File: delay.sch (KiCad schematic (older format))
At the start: 19 parts, among them U201 PT2399

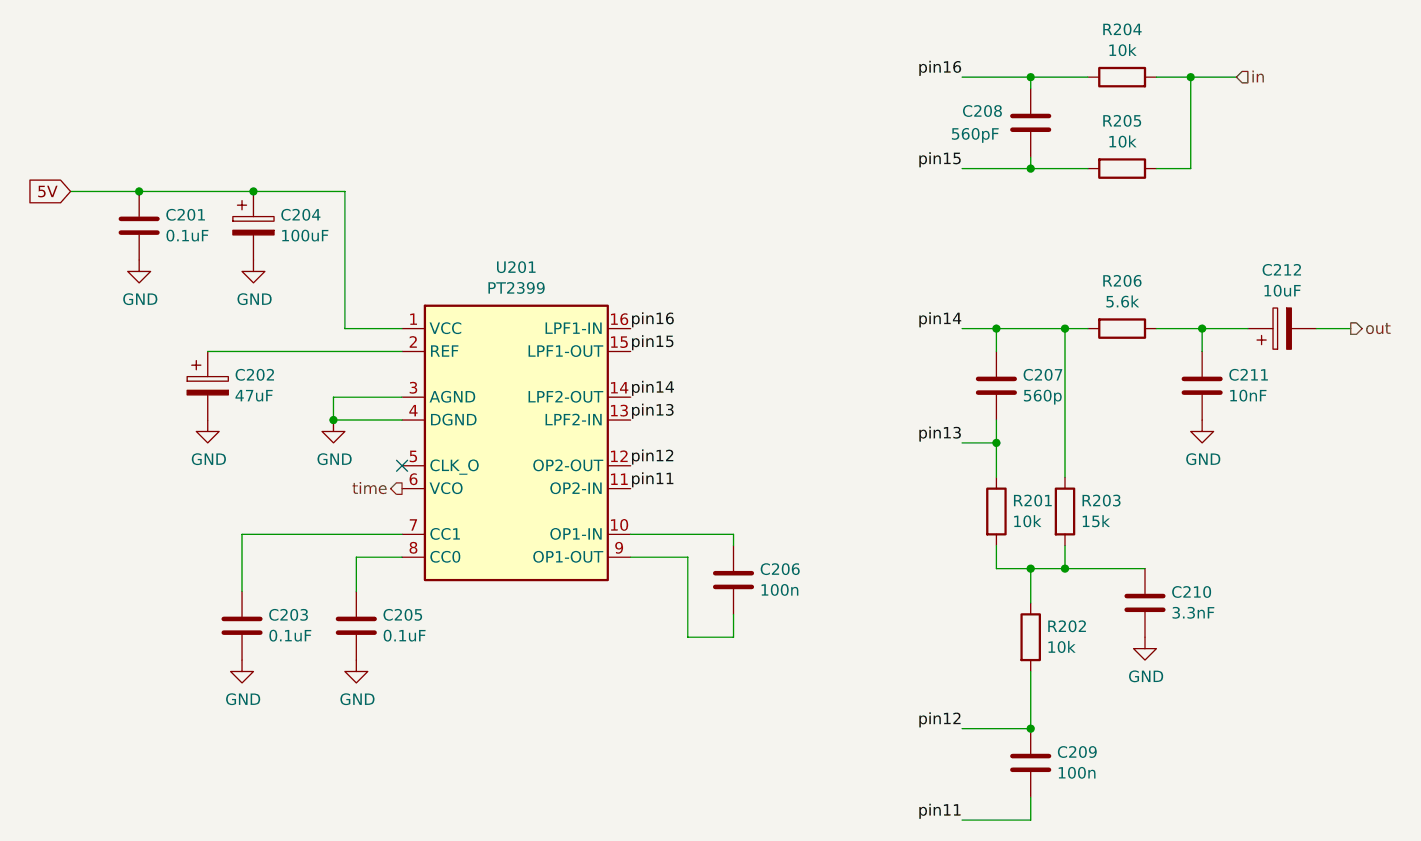
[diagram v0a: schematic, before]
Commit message: Clipping diodes work
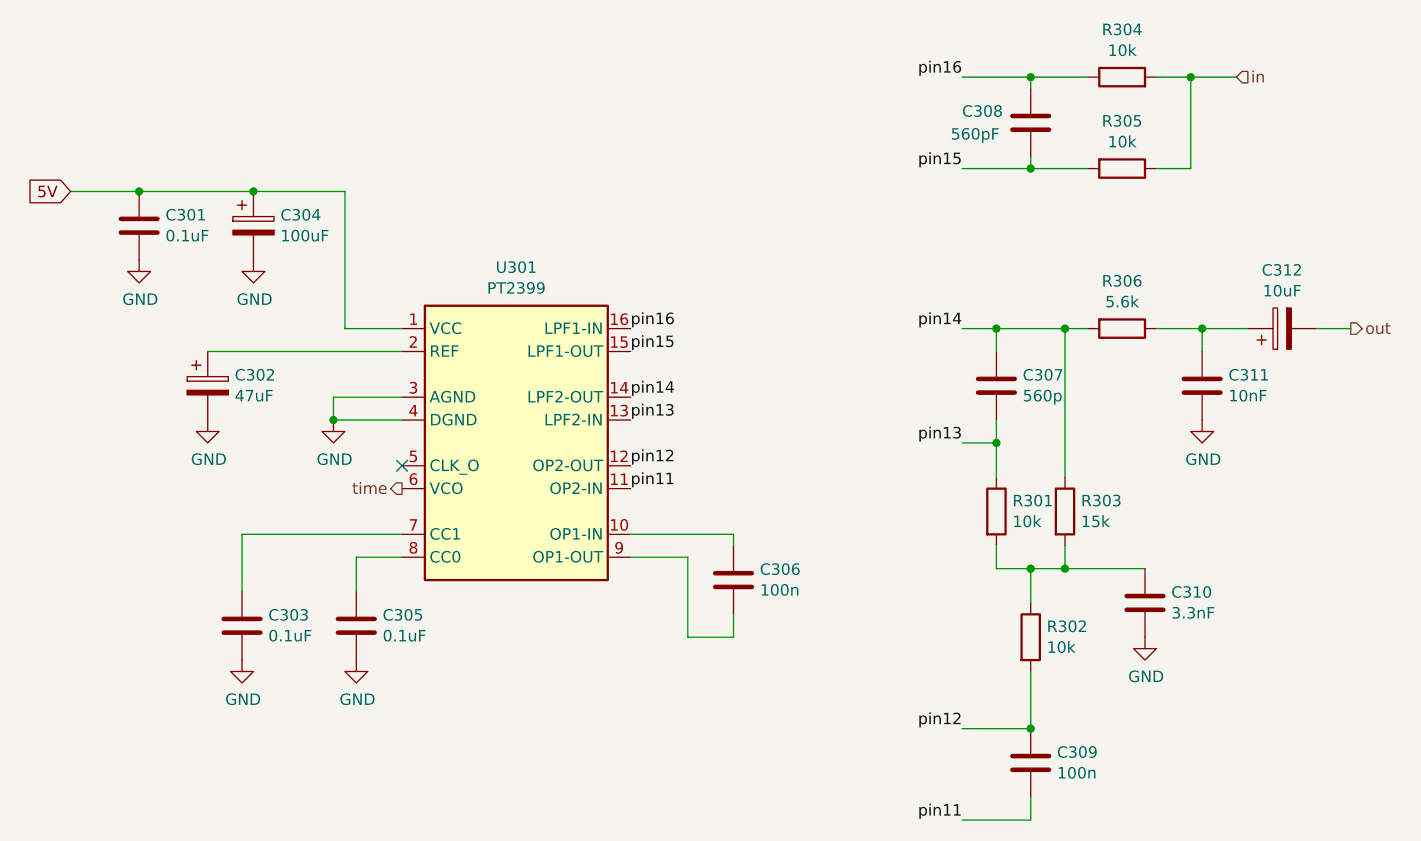
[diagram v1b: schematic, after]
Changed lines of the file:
@@
 AR Path="/5F90D1E6/5F9242A3" Ref="U201"  Part="1"
 AR Path="/5F9672E5/5F9242A3" Ref="U301"  Part="1"
-F 0 "U201" H 3700 4267 50  0000 C CNN
+F 0 "U301" H 3700 4267 50  0000 C CNN
 F 1 "PT2399" H 3700 4176 50  0000 C CNN
 F 2 "" H 3700 3100 50  0001 C CNN
@@
 AR Path="/5F90D1E6/5F9242A9" Ref="C203"  Part="1"
 AR Path="/5F9672E5/5F9242A9" Ref="C303"  Part="1"
-F 0 "C203" H 2615 4346 50  0000 L CNN
+F 0 "C303" H 2615 4346 50  0000 L CNN
 F 1 "0.1uF" H 2615 4255 50  0000 L CNN
 F 2 "" H 2538 4150 50  0001 C CNN
@@
 AR Path="/5F90D1E6/5F9242AF" Ref="C205"  Part="1"
 AR Path="/5F9672E5/5F9242AF" Ref="C305"  Part="1"
-F 0 "C205" H 3115 4346 50  0000 L CNN
+F 0 "C305" H 3115 4346 50  0000 L CNN
 F 1 "0.1uF" H 3115 4255 50  0000 L CNN
 F 2 "" H 3038 4150 50  0001 C CNN
@@
 AR Path="/5F90D1E6/5F9242B9" Ref="#PWR0204"  Part="1"
 AR Path="/5F9672E5/5F9242B9" Ref="#PWR0304"  Part="1"
-F 0 "#PWR0204" H 2500 4200 50  0001 C CNN
+F 0 "#PWR0304" H 2500 4200 50  0001 C CNN
 F 1 "GND" H 2505 4277 50  0000 C CNN
 F 2 "" H 2500 4450 50  0001 C CNN
@@
 AR Path="/5F90D1E6/5F9242BF" Ref="#PWR0207"  Part="1"
 AR Path="/5F9672E5/5F9242BF" Ref="#PWR0307"  Part="1"
-F 0 "#PWR0207" H 3000 4200 50  0001 C CNN
+F 0 "#PWR0307" H 3000 4200 50  0001 C CNN
 F 1 "GND" H 3005 4277 50  0000 C CNN
 F 2 "" H 3000 4450 50  0001 C CNN
@@
 AR Path="/5F90D1E6/5F9242C5" Ref="C201"  Part="1"
 AR Path="/5F9672E5/5F9242C5" Ref="C301"  Part="1"
-F 0 "C201" H 2165 2596 50  0000 L CNN
+F 0 "C301" H 2165 2596 50  0000 L CNN
 F 1 "0.1uF" H 2165 2505 50  0000 L CNN
 F 2 "" H 2088 2400 50  0001 C CNN
@@
 AR Path="/5F90D1E6/5F9242CB" Ref="C204"  Part="1"
 AR Path="/5F9672E5/5F9242CB" Ref="C304"  Part="1"
-F 0 "C204" H 2668 2596 50  0000 L CNN
+F 0 "C304" H 2668 2596 50  0000 L CNN
 F 1 "100uF" H 2668 2505 50  0000 L CNN
 F 2 "" H 2588 2400 50  0001 C CNN
@@
 AR Path="/5F90D1E6/5F9242D4" Ref="#PWR0202"  Part="1"
 AR Path="/5F9672E5/5F9242D4" Ref="#PWR0302"  Part="1"
-F 0 "#PWR0202" H 2050 2450 50  0001 C CNN
+F 0 "#PWR0302" H 2050 2450 50  0001 C CNN
 F 1 "GND" H 2055 2527 50  0000 C CNN
 F 2 "" H 2050 2700 50  0001 C CNN
@@
 AR Path="/5F90D1E6/5F9242DA" Ref="#PWR0205"  Part="1"
 AR Path="/5F9672E5/5F9242DA" Ref="#PWR0305"  Part="1"
-F 0 "#PWR0205" H 2550 2450 50  0001 C CNN
+F 0 "#PWR0305" H 2550 2450 50  0001 C CNN
 F 1 "GND" H 2555 2527 50  0000 C CNN
 F 2 "" H 2550 2700 50  0001 C CNN
@@
 AR Path="/5F90D1E6/5F9242E4" Ref="C202"  Part="1"
 AR Path="/5F9672E5/5F9242E4" Ref="C302"  Part="1"
-F 0 "C202" H 2468 3296 50  0000 L CNN
+F 0 "C302" H 2468 3296 50  0000 L CNN
 F 1 "47uF" H 2468 3205 50  0000 L CNN
 F 2 "" H 2388 3100 50  0001 C CNN
@@
 AR Path="/5F90D1E6/5F9242EA" Ref="#PWR0203"  Part="1"
 AR Path="/5F9672E5/5F9242EA" Ref="#PWR0303"  Part="1"
-F 0 "#PWR0203" H 2350 3150 50  0001 C CNN
+F 0 "#PWR0303" H 2350 3150 50  0001 C CNN
 F 1 "GND" H 2355 3227 50  0000 C CNN
 F 2 "" H 2350 3400 50  0001 C CNN
@@
 AR Path="/5F90D1E6/5F9242F9" Ref="C206"  Part="1"
 AR Path="/5F9672E5/5F9242F9" Ref="C306"  Part="1"
-F 0 "C206" H 4765 4146 50  0000 L CNN
+F 0 "C306" H 4765 4146 50  0000 L CNN
 F 1 "100n" H 4765 4055 50  0000 L CNN
 F 2 "" H 4688 3950 50  0001 C CNN
@@
 AR Path="/5F90D1E6/5F924306" Ref="#PWR0206"  Part="1"
 AR Path="/5F9672E5/5F924306" Ref="#PWR0306"  Part="1"
-F 0 "#PWR0206" H 2900 3150 50  0001 C CNN
+F 0 "#PWR0306" H 2900 3150 50  0001 C CNN
 F 1 "GND" H 2905 3227 50  0000 C CNN
 F 2 "" H 2900 3400 50  0001 C CNN
@@
 AR Path="/5F90D1E6/5F934513" Ref="C208"  Part="1"
 AR Path="/5F9672E5/5F934513" Ref="C308"  Part="1"
-F 0 "C208" H 5650 2150 50  0000 L CNN
+F 0 "C308" H 5650 2150 50  0000 L CNN
 F 1 "560pF" H 5600 2050 50  0000 L CNN
 F 2 "" H 5988 1950 50  0001 C CNN
@@
 AR Path="/5F90D1E6/5F934519" Ref="R204"  Part="1"
 AR Path="/5F9672E5/5F934519" Ref="R304"  Part="1"
-F 0 "R204" V 6557 1900 50  0000 C CNN
+F 0 "R304" V 6557 1900 50  0000 C CNN
 F 1 "10k" V 6466 1900 50  0000 C CNN
 F 2 "" V 6280 1900 50  0001 C CNN
@@
 AR Path="/5F90D1E6/5F93451F" Ref="R205"  Part="1"
 AR Path="/5F9672E5/5F93451F" Ref="R305"  Part="1"
-F 0 "R205" V 6143 2300 50  0000 C CNN
+F 0 "R305" V 6143 2300 50  0000 C CNN
 F 1 "10k" V 6234 2300 50  0000 C CNN
 F 2 "" V 6280 2300 50  0001 C CNN
@@
 AR Path="/5F90D1E6/5F934560" Ref="R206"  Part="1"
 AR Path="/5F9672E5/5F934560" Ref="R306"  Part="1"
-F 0 "R206" V 6143 3000 50  0000 C CNN
+F 0 "R306" V 6143 3000 50  0000 C CNN
 F 1 "5.6k" V 6234 3000 50  0000 C CNN
 F 2 "" V 6280 3000 50  0001 C CNN
@@
 AR Path="/5F90D1E6/5F934566" Ref="C211"  Part="1"
 AR Path="/5F9672E5/5F934566" Ref="C311"  Part="1"
-F 0 "C211" H 6815 3296 50  0000 L CNN
+F 0 "C311" H 6815 3296 50  0000 L CNN
 F 1 "10nF" H 6815 3205 50  0000 L CNN
 F 2 "" H 6738 3100 50  0001 C CNN
@@
 AR Path="/5F90D1E6/5F93456C" Ref="C212"  Part="1"
 AR Path="/5F9672E5/5F93456C" Ref="C312"  Part="1"
-F 0 "C212" V 7305 3000 50  0000 C CNN
+F 0 "C312" V 7305 3000 50  0000 C CNN
 F 1 "10uF" V 7214 3000 50  0000 C CNN
 F 2 "" H 7088 2850 50  0001 C CNN
@@
 AR Path="/5F90D1E6/5F93457D" Ref="#PWR0209"  Part="1"
 AR Path="/5F9672E5/5F93457D" Ref="#PWR0309"  Part="1"
-F 0 "#PWR0209" H 6700 3150 50  0001 C CNN
+F 0 "#PWR0309" H 6700 3150 50  0001 C CNN
 F 1 "GND" H 6705 3227 50  0000 C CNN
 F 2 "" H 6700 3400 50  0001 C CNN
@@
 AR Path="/5F90D1E6/5F93458D" Ref="C207"  Part="1"
 AR Path="/5F9672E5/5F93458D" Ref="C307"  Part="1"
-F 0 "C207" H 5915 3296 50  0000 L CNN
+F 0 "C307" H 5915 3296 50  0000 L CNN
 F 1 "560p" H 5915 3205 50  0000 L CNN
 F 2 "" H 5838 3100 50  0001 C CNN
@@
 AR Path="/5F90D1E6/5F93459C" Ref="R203"  Part="1"
 AR Path="/5F9672E5/5F93459C" Ref="R303"  Part="1"
-F 0 "R203" H 6170 3846 50  0000 L CNN
+F 0 "R303" H 6170 3846 50  0000 L CNN
 F 1 "15k" H 6170 3755 50  0000 L CNN
 F 2 "" V 6030 3800 50  0001 C CNN
@@
 AR Path="/5F90D1E6/5F9345A2" Ref="R201"  Part="1"
 AR Path="/5F9672E5/5F9345A2" Ref="R301"  Part="1"
-F 0 "R201" H 5870 3846 50  0000 L CNN
+F 0 "R301" H 5870 3846 50  0000 L CNN
 F 1 "10k" H 5870 3755 50  0000 L CNN
 F 2 "" V 5730 3800 50  0001 C CNN
@@
 AR Path="/5F90D1E6/5F9345AD" Ref="C210"  Part="1"
 AR Path="/5F9672E5/5F9345AD" Ref="C310"  Part="1"
-F 0 "C210" H 6565 4246 50  0000 L CNN
+F 0 "C310" H 6565 4246 50  0000 L CNN
 F 1 "3.3nF" H 6565 4155 50  0000 L CNN
 F 2 "" H 6488 4050 50  0001 C CNN
@@
 AR Path="/5F90D1E6/5F9345B3" Ref="#PWR0208"  Part="1"
 AR Path="/5F9672E5/5F9345B3" Ref="#PWR0308"  Part="1"
-F 0 "#PWR0208" H 6450 4100 50  0001 C CNN
+F 0 "#PWR0308" H 6450 4100 50  0001 C CNN
 F 1 "GND" H 6455 4177 50  0000 C CNN
 F 2 "" H 6450 4350 50  0001 C CNN
@@
 AR Path="/5F90D1E6/5F9345BB" Ref="R202"  Part="1"
 AR Path="/5F9672E5/5F9345BB" Ref="R302"  Part="1"
-F 0 "R202" H 6020 4396 50  0000 L CNN
+F 0 "R302" H 6020 4396 50  0000 L CNN
 F 1 "10k" H 6020 4305 50  0000 L CNN
 F 2 "" V 5880 4350 50  0001 C CNN
@@
 AR Path="/5F90D1E6/5F9345C6" Ref="C209"  Part="1"
 AR Path="/5F9672E5/5F9345C6" Ref="C309"  Part="1"
-F 0 "C209" H 6065 4946 50  0000 L CNN
+F 0 "C309" H 6065 4946 50  0000 L CNN
 F 1 "100n" H 6065 4855 50  0000 L CNN
 F 2 "" H 5988 4750 50  0001 C CNN

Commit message: lmao
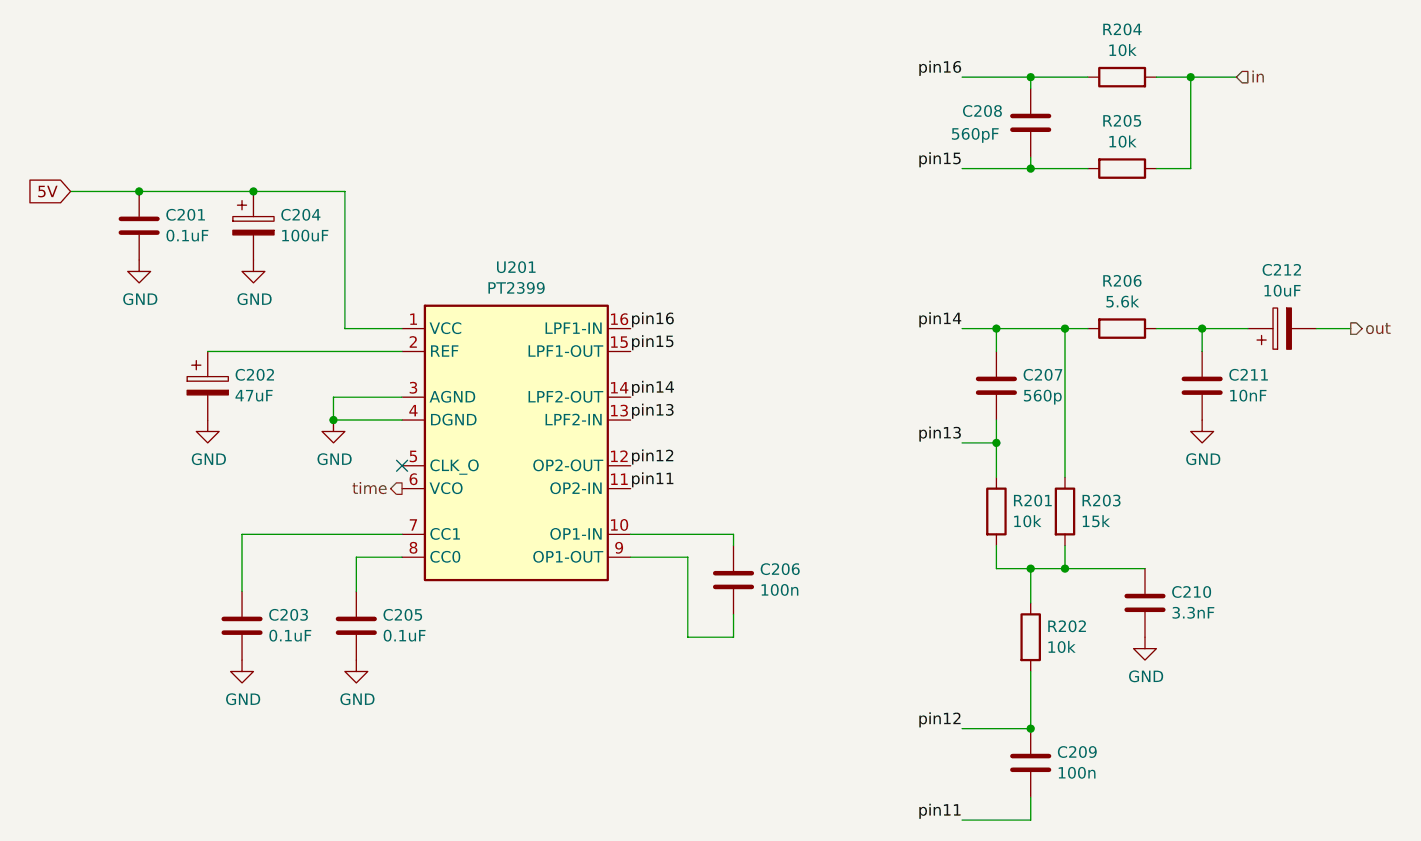
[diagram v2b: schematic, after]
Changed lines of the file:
@@
 AR Path="/5F90D1E6/5F9242A3" Ref="U201"  Part="1"
 AR Path="/5F9672E5/5F9242A3" Ref="U301"  Part="1"
-F 0 "U301" H 3700 4267 50  0000 C CNN
+F 0 "U201" H 3700 4267 50  0000 C CNN
 F 1 "PT2399" H 3700 4176 50  0000 C CNN
 F 2 "" H 3700 3100 50  0001 C CNN
@@
 AR Path="/5F90D1E6/5F9242A9" Ref="C203"  Part="1"
 AR Path="/5F9672E5/5F9242A9" Ref="C303"  Part="1"
-F 0 "C303" H 2615 4346 50  0000 L CNN
+F 0 "C203" H 2615 4346 50  0000 L CNN
 F 1 "0.1uF" H 2615 4255 50  0000 L CNN
 F 2 "" H 2538 4150 50  0001 C CNN
@@
 AR Path="/5F90D1E6/5F9242AF" Ref="C205"  Part="1"
 AR Path="/5F9672E5/5F9242AF" Ref="C305"  Part="1"
-F 0 "C305" H 3115 4346 50  0000 L CNN
+F 0 "C205" H 3115 4346 50  0000 L CNN
 F 1 "0.1uF" H 3115 4255 50  0000 L CNN
 F 2 "" H 3038 4150 50  0001 C CNN
@@
 AR Path="/5F90D1E6/5F9242B9" Ref="#PWR0204"  Part="1"
 AR Path="/5F9672E5/5F9242B9" Ref="#PWR0304"  Part="1"
-F 0 "#PWR0304" H 2500 4200 50  0001 C CNN
+F 0 "#PWR0204" H 2500 4200 50  0001 C CNN
 F 1 "GND" H 2505 4277 50  0000 C CNN
 F 2 "" H 2500 4450 50  0001 C CNN
@@
 AR Path="/5F90D1E6/5F9242BF" Ref="#PWR0207"  Part="1"
 AR Path="/5F9672E5/5F9242BF" Ref="#PWR0307"  Part="1"
-F 0 "#PWR0307" H 3000 4200 50  0001 C CNN
+F 0 "#PWR0207" H 3000 4200 50  0001 C CNN
 F 1 "GND" H 3005 4277 50  0000 C CNN
 F 2 "" H 3000 4450 50  0001 C CNN
@@
 AR Path="/5F90D1E6/5F9242C5" Ref="C201"  Part="1"
 AR Path="/5F9672E5/5F9242C5" Ref="C301"  Part="1"
-F 0 "C301" H 2165 2596 50  0000 L CNN
+F 0 "C201" H 2165 2596 50  0000 L CNN
 F 1 "0.1uF" H 2165 2505 50  0000 L CNN
 F 2 "" H 2088 2400 50  0001 C CNN
@@
 AR Path="/5F90D1E6/5F9242CB" Ref="C204"  Part="1"
 AR Path="/5F9672E5/5F9242CB" Ref="C304"  Part="1"
-F 0 "C304" H 2668 2596 50  0000 L CNN
+F 0 "C204" H 2668 2596 50  0000 L CNN
 F 1 "100uF" H 2668 2505 50  0000 L CNN
 F 2 "" H 2588 2400 50  0001 C CNN
@@
 AR Path="/5F90D1E6/5F9242D4" Ref="#PWR0202"  Part="1"
 AR Path="/5F9672E5/5F9242D4" Ref="#PWR0302"  Part="1"
-F 0 "#PWR0302" H 2050 2450 50  0001 C CNN
+F 0 "#PWR0202" H 2050 2450 50  0001 C CNN
 F 1 "GND" H 2055 2527 50  0000 C CNN
 F 2 "" H 2050 2700 50  0001 C CNN
@@
 AR Path="/5F90D1E6/5F9242DA" Ref="#PWR0205"  Part="1"
 AR Path="/5F9672E5/5F9242DA" Ref="#PWR0305"  Part="1"
-F 0 "#PWR0305" H 2550 2450 50  0001 C CNN
+F 0 "#PWR0205" H 2550 2450 50  0001 C CNN
 F 1 "GND" H 2555 2527 50  0000 C CNN
 F 2 "" H 2550 2700 50  0001 C CNN
@@
 AR Path="/5F90D1E6/5F9242E4" Ref="C202"  Part="1"
 AR Path="/5F9672E5/5F9242E4" Ref="C302"  Part="1"
-F 0 "C302" H 2468 3296 50  0000 L CNN
+F 0 "C202" H 2468 3296 50  0000 L CNN
 F 1 "47uF" H 2468 3205 50  0000 L CNN
 F 2 "" H 2388 3100 50  0001 C CNN
@@
 AR Path="/5F90D1E6/5F9242EA" Ref="#PWR0203"  Part="1"
 AR Path="/5F9672E5/5F9242EA" Ref="#PWR0303"  Part="1"
-F 0 "#PWR0303" H 2350 3150 50  0001 C CNN
+F 0 "#PWR0203" H 2350 3150 50  0001 C CNN
 F 1 "GND" H 2355 3227 50  0000 C CNN
 F 2 "" H 2350 3400 50  0001 C CNN
@@
 AR Path="/5F90D1E6/5F9242F9" Ref="C206"  Part="1"
 AR Path="/5F9672E5/5F9242F9" Ref="C306"  Part="1"
-F 0 "C306" H 4765 4146 50  0000 L CNN
+F 0 "C206" H 4765 4146 50  0000 L CNN
 F 1 "100n" H 4765 4055 50  0000 L CNN
 F 2 "" H 4688 3950 50  0001 C CNN
@@
 AR Path="/5F90D1E6/5F924306" Ref="#PWR0206"  Part="1"
 AR Path="/5F9672E5/5F924306" Ref="#PWR0306"  Part="1"
-F 0 "#PWR0306" H 2900 3150 50  0001 C CNN
+F 0 "#PWR0206" H 2900 3150 50  0001 C CNN
 F 1 "GND" H 2905 3227 50  0000 C CNN
 F 2 "" H 2900 3400 50  0001 C CNN
@@
 AR Path="/5F90D1E6/5F934513" Ref="C208"  Part="1"
 AR Path="/5F9672E5/5F934513" Ref="C308"  Part="1"
-F 0 "C308" H 5650 2150 50  0000 L CNN
+F 0 "C208" H 5650 2150 50  0000 L CNN
 F 1 "560pF" H 5600 2050 50  0000 L CNN
 F 2 "" H 5988 1950 50  0001 C CNN
@@
 AR Path="/5F90D1E6/5F934519" Ref="R204"  Part="1"
 AR Path="/5F9672E5/5F934519" Ref="R304"  Part="1"
-F 0 "R304" V 6557 1900 50  0000 C CNN
+F 0 "R204" V 6557 1900 50  0000 C CNN
 F 1 "10k" V 6466 1900 50  0000 C CNN
 F 2 "" V 6280 1900 50  0001 C CNN
@@
 AR Path="/5F90D1E6/5F93451F" Ref="R205"  Part="1"
 AR Path="/5F9672E5/5F93451F" Ref="R305"  Part="1"
-F 0 "R305" V 6143 2300 50  0000 C CNN
+F 0 "R205" V 6143 2300 50  0000 C CNN
 F 1 "10k" V 6234 2300 50  0000 C CNN
 F 2 "" V 6280 2300 50  0001 C CNN
@@
 AR Path="/5F90D1E6/5F934560" Ref="R206"  Part="1"
 AR Path="/5F9672E5/5F934560" Ref="R306"  Part="1"
-F 0 "R306" V 6143 3000 50  0000 C CNN
+F 0 "R206" V 6143 3000 50  0000 C CNN
 F 1 "5.6k" V 6234 3000 50  0000 C CNN
 F 2 "" V 6280 3000 50  0001 C CNN
@@
 AR Path="/5F90D1E6/5F934566" Ref="C211"  Part="1"
 AR Path="/5F9672E5/5F934566" Ref="C311"  Part="1"
-F 0 "C311" H 6815 3296 50  0000 L CNN
+F 0 "C211" H 6815 3296 50  0000 L CNN
 F 1 "10nF" H 6815 3205 50  0000 L CNN
 F 2 "" H 6738 3100 50  0001 C CNN
@@
 AR Path="/5F90D1E6/5F93456C" Ref="C212"  Part="1"
 AR Path="/5F9672E5/5F93456C" Ref="C312"  Part="1"
-F 0 "C312" V 7305 3000 50  0000 C CNN
+F 0 "C212" V 7305 3000 50  0000 C CNN
 F 1 "10uF" V 7214 3000 50  0000 C CNN
 F 2 "" H 7088 2850 50  0001 C CNN
@@
 AR Path="/5F90D1E6/5F93457D" Ref="#PWR0209"  Part="1"
 AR Path="/5F9672E5/5F93457D" Ref="#PWR0309"  Part="1"
-F 0 "#PWR0309" H 6700 3150 50  0001 C CNN
+F 0 "#PWR0209" H 6700 3150 50  0001 C CNN
 F 1 "GND" H 6705 3227 50  0000 C CNN
 F 2 "" H 6700 3400 50  0001 C CNN
@@
 AR Path="/5F90D1E6/5F93458D" Ref="C207"  Part="1"
 AR Path="/5F9672E5/5F93458D" Ref="C307"  Part="1"
-F 0 "C307" H 5915 3296 50  0000 L CNN
+F 0 "C207" H 5915 3296 50  0000 L CNN
 F 1 "560p" H 5915 3205 50  0000 L CNN
 F 2 "" H 5838 3100 50  0001 C CNN
@@
 AR Path="/5F90D1E6/5F93459C" Ref="R203"  Part="1"
 AR Path="/5F9672E5/5F93459C" Ref="R303"  Part="1"
-F 0 "R303" H 6170 3846 50  0000 L CNN
+F 0 "R203" H 6170 3846 50  0000 L CNN
 F 1 "15k" H 6170 3755 50  0000 L CNN
 F 2 "" V 6030 3800 50  0001 C CNN
@@
 AR Path="/5F90D1E6/5F9345A2" Ref="R201"  Part="1"
 AR Path="/5F9672E5/5F9345A2" Ref="R301"  Part="1"
-F 0 "R301" H 5870 3846 50  0000 L CNN
+F 0 "R201" H 5870 3846 50  0000 L CNN
 F 1 "10k" H 5870 3755 50  0000 L CNN
 F 2 "" V 5730 3800 50  0001 C CNN
@@
 AR Path="/5F90D1E6/5F9345AD" Ref="C210"  Part="1"
 AR Path="/5F9672E5/5F9345AD" Ref="C310"  Part="1"
-F 0 "C310" H 6565 4246 50  0000 L CNN
+F 0 "C210" H 6565 4246 50  0000 L CNN
 F 1 "3.3nF" H 6565 4155 50  0000 L CNN
 F 2 "" H 6488 4050 50  0001 C CNN
@@
 AR Path="/5F90D1E6/5F9345B3" Ref="#PWR0208"  Part="1"
 AR Path="/5F9672E5/5F9345B3" Ref="#PWR0308"  Part="1"
-F 0 "#PWR0308" H 6450 4100 50  0001 C CNN
+F 0 "#PWR0208" H 6450 4100 50  0001 C CNN
 F 1 "GND" H 6455 4177 50  0000 C CNN
 F 2 "" H 6450 4350 50  0001 C CNN
@@
 AR Path="/5F90D1E6/5F9345BB" Ref="R202"  Part="1"
 AR Path="/5F9672E5/5F9345BB" Ref="R302"  Part="1"
-F 0 "R302" H 6020 4396 50  0000 L CNN
+F 0 "R202" H 6020 4396 50  0000 L CNN
 F 1 "10k" H 6020 4305 50  0000 L CNN
 F 2 "" V 5880 4350 50  0001 C CNN
@@
 AR Path="/5F90D1E6/5F9345C6" Ref="C209"  Part="1"
 AR Path="/5F9672E5/5F9345C6" Ref="C309"  Part="1"
-F 0 "C309" H 6065 4946 50  0000 L CNN
+F 0 "C209" H 6065 4946 50  0000 L CNN
 F 1 "100n" H 6065 4855 50  0000 L CNN
 F 2 "" H 5988 4750 50  0001 C CNN
